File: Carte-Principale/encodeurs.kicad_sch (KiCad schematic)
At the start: 9 parts, among them J8 Encodeur_G, J9 Encodeur_D, U2 AM26LV32xD

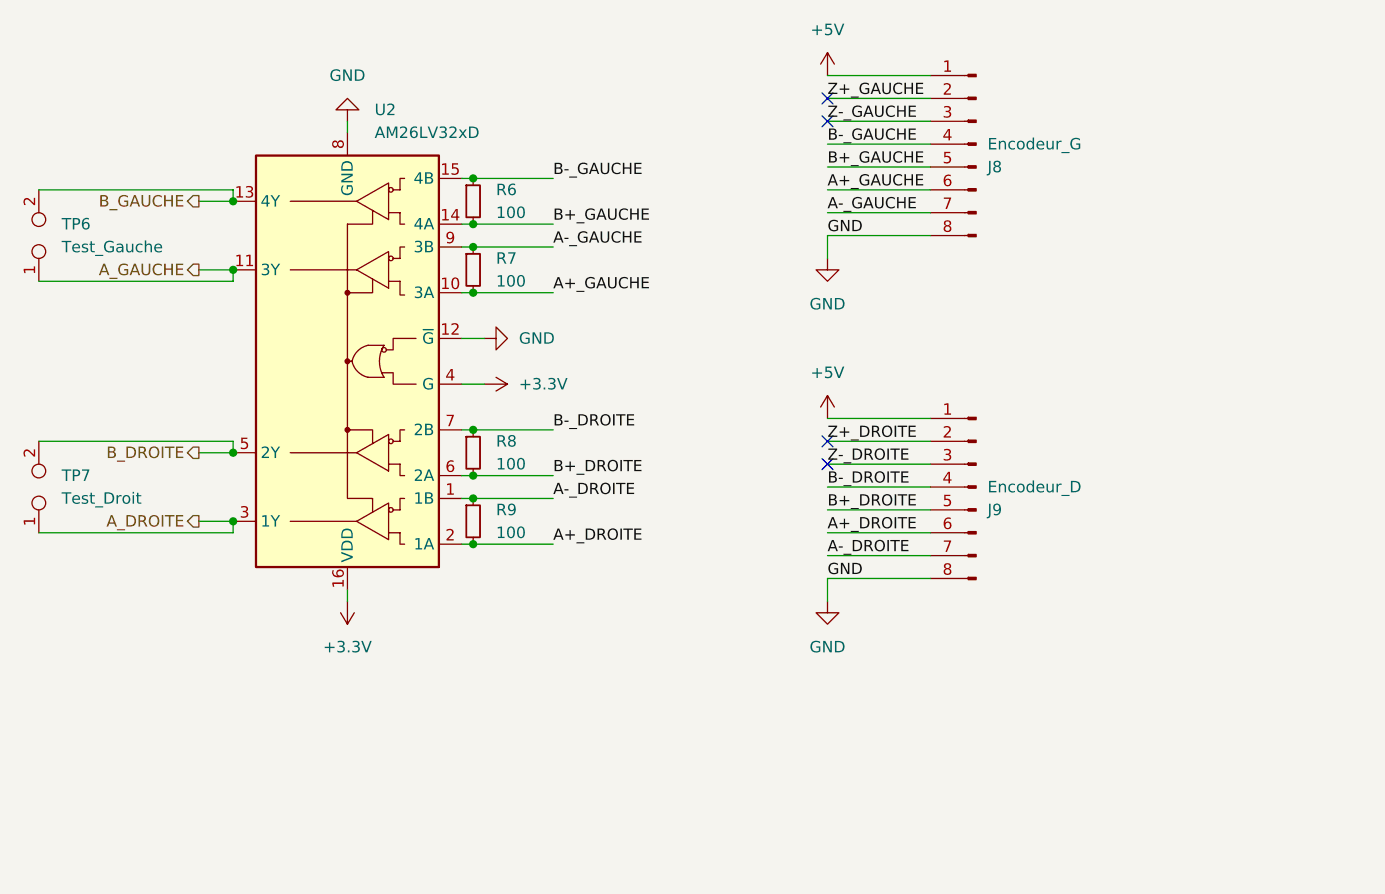
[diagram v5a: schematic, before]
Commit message: avancée
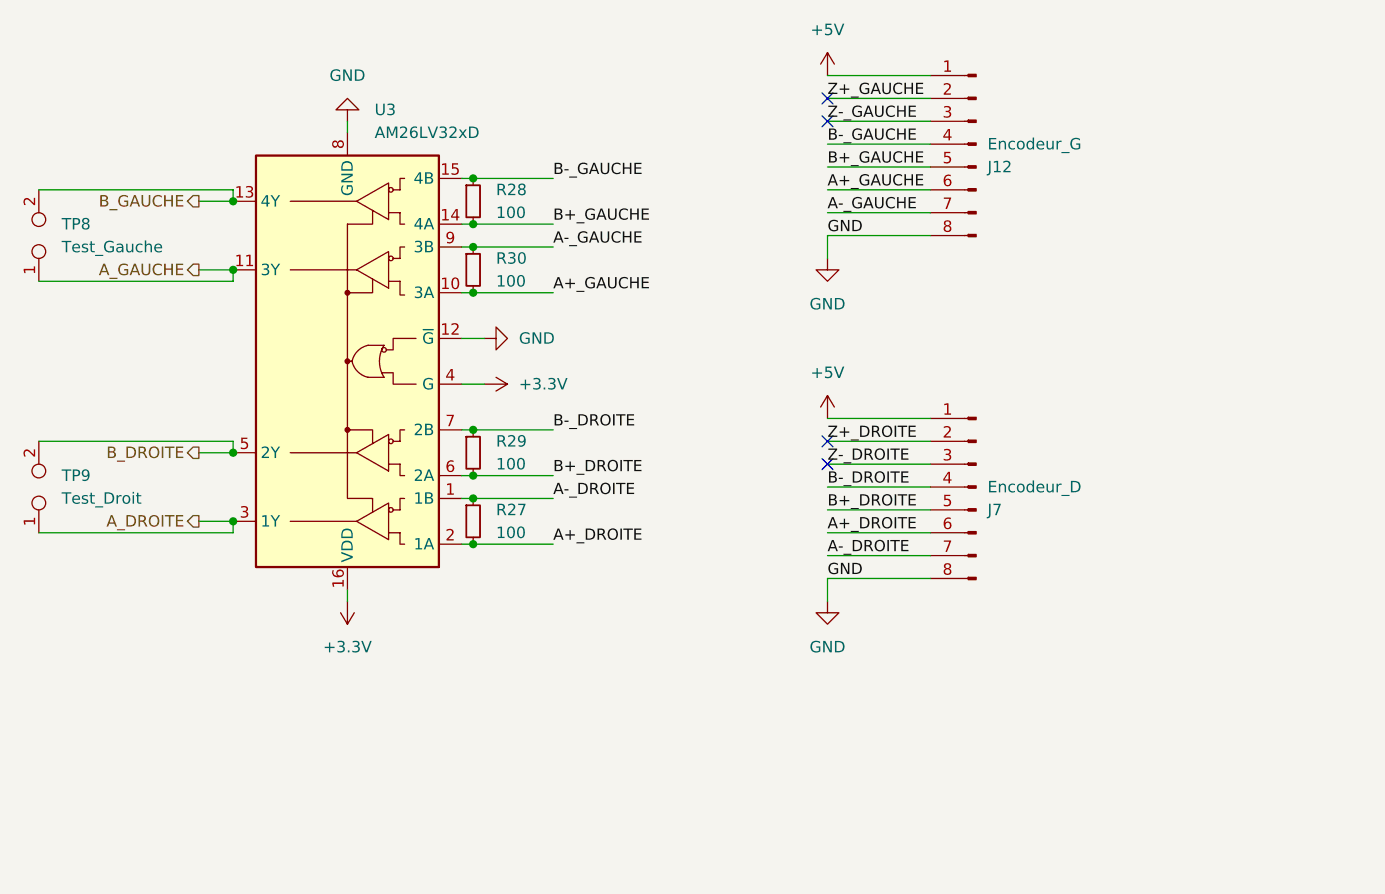
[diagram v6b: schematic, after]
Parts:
- renumbered J8 to J12, J9 to J7, R9 to R27, R6 to R28, R8 to R29, R7 to R30, TP6 to TP8, TP7 to TP9, U2 to U3
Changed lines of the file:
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@@
 		(dnp no)
 		(fields_autoplaced yes)
-		(property "Reference" "TP7"
+		(property "Reference" "TP9"
 			(at 40.64 77.4699 90)
 			(effects
@@
 			(project "Carte-Principale"
 				(path "/88b0dd29-ac24-4c5d-804c-fc642ecf6263/a2923913-7939-4f75-8694-93f1ab74a018"
-					(reference "TP7")
+					(reference "TP9")
 					(unit 1)
 				)
@@
 		(dnp no)
 		(fields_autoplaced yes)
-		(property "Reference" "J9"
+		(property "Reference" "J7"
 			(at 143.51 81.2801 0)
 			(effects
@@
 			(project "Carte-Principale"
 				(path "/88b0dd29-ac24-4c5d-804c-fc642ecf6263/a2923913-7939-4f75-8694-93f1ab74a018"
-					(reference "J9")
+					(reference "J7")
 					(unit 1)
 				)
@@
 		(dnp no)
 		(fields_autoplaced yes)
-		(property "Reference" "TP6"
+		(property "Reference" "TP8"
 			(at 40.64 49.5299 90)
 			(effects
@@
 			(project "Carte-Principale"
 				(path "/88b0dd29-ac24-4c5d-804c-fc642ecf6263/a2923913-7939-4f75-8694-93f1ab74a018"
-					(reference "TP6")
+					(reference "TP8")
 					(unit 1)
 				)
@@
 		(dnp no)
 		(fields_autoplaced yes)
-		(property "Reference" "R8"
+		(property "Reference" "R29"
 			(at 88.9 73.6599 0)
 			(effects
@@
 			(project "Carte-Principale"
 				(path "/88b0dd29-ac24-4c5d-804c-fc642ecf6263/a2923913-7939-4f75-8694-93f1ab74a018"
-					(reference "R8")
+					(reference "R29")
 					(unit 1)
 				)
@@
 		(dnp no)
 		(fields_autoplaced yes)
-		(property "Reference" "R7"
+		(property "Reference" "R30"
 			(at 88.9 53.3399 0)
 			(effects
@@
 			(project "Carte-Principale"
 				(path "/88b0dd29-ac24-4c5d-804c-fc642ecf6263/a2923913-7939-4f75-8694-93f1ab74a018"
-					(reference "R7")
+					(reference "R30")
 					(unit 1)
 				)
@@
 		(dnp no)
 		(fields_autoplaced yes)
-		(property "Reference" "J8"
+		(property "Reference" "J12"
 			(at 143.51 43.1801 0)
 			(effects
@@
 			(project "Carte-Principale"
 				(path "/88b0dd29-ac24-4c5d-804c-fc642ecf6263/a2923913-7939-4f75-8694-93f1ab74a018"
-					(reference "J8")
+					(reference "J12")
 					(unit 1)
 				)
@@
 		(dnp no)
 		(fields_autoplaced yes)
-		(property "Reference" "R6"
+		(property "Reference" "R28"
 			(at 88.9 45.7199 0)
 			(effects
@@
 			(project "Carte-Principale"
 				(path "/88b0dd29-ac24-4c5d-804c-fc642ecf6263/a2923913-7939-4f75-8694-93f1ab74a018"
-					(reference "R6")
+					(reference "R28")
 					(unit 1)
 				)
@@
 		(dnp no)
 		(fields_autoplaced yes)
-		(property "Reference" "R9"
+		(property "Reference" "R27"
 			(at 88.9 81.2799 0)
 			(effects
@@
 			(project "Carte-Principale"
 				(path "/88b0dd29-ac24-4c5d-804c-fc642ecf6263/a2923913-7939-4f75-8694-93f1ab74a018"
-					(reference "R9")
+					(reference "R27")
 					(unit 1)
 				)
@@
 		(dnp no)
 		(fields_autoplaced yes)
-		(property "Reference" "U2"
+		(property "Reference" "U3"
 			(at 75.4065 36.83 0)
 			(effects
@@
 			(project "Carte-Principale"
 				(path "/88b0dd29-ac24-4c5d-804c-fc642ecf6263/a2923913-7939-4f75-8694-93f1ab74a018"
-					(reference "U2")
-					(unit 1)
-				)
+					(reference "U3")
+					(unit 1)
+				)

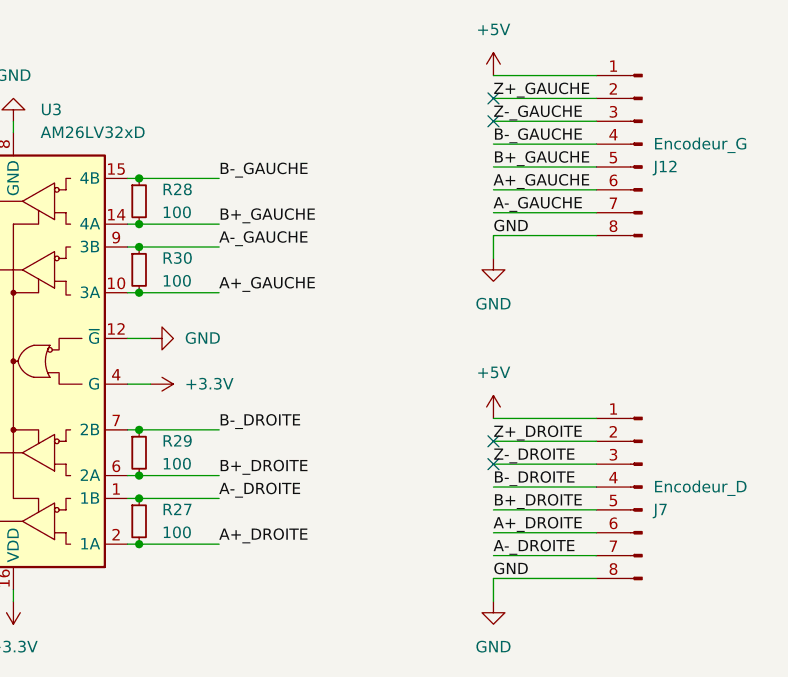
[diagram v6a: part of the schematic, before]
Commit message: Final pcb modification
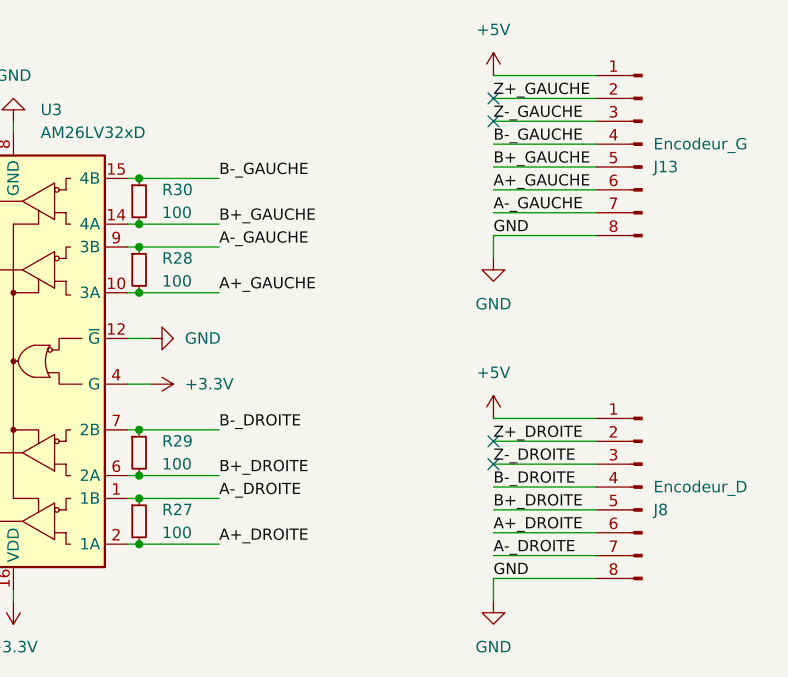
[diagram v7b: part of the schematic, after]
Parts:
- renumbered J12 to J13, J7 to J8, R30 to R28, R28 to R30
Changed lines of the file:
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@@
 		(dnp no)
 		(fields_autoplaced yes)
-		(property "Reference" "J7"
+		(property "Reference" "J8"
 			(at 143.51 81.2801 0)
 			(effects
@@
 			(project "Carte-Principale"
 				(path "/88b0dd29-ac24-4c5d-804c-fc642ecf6263/a2923913-7939-4f75-8694-93f1ab74a018"
-					(reference "J7")
+					(reference "J8")
 					(unit 1)
 				)
@@
 		(dnp no)
 		(fields_autoplaced yes)
-		(property "Reference" "R30"
+		(property "Reference" "R28"
 			(at 88.9 53.3399 0)
 			(effects
@@
 			(project "Carte-Principale"
 				(path "/88b0dd29-ac24-4c5d-804c-fc642ecf6263/a2923913-7939-4f75-8694-93f1ab74a018"
-					(reference "R30")
+					(reference "R28")
 					(unit 1)
 				)
@@
 		(dnp no)
 		(fields_autoplaced yes)
-		(property "Reference" "J12"
+		(property "Reference" "J13"
 			(at 143.51 43.1801 0)
 			(effects
@@
 			(project "Carte-Principale"
 				(path "/88b0dd29-ac24-4c5d-804c-fc642ecf6263/a2923913-7939-4f75-8694-93f1ab74a018"
-					(reference "J12")
+					(reference "J13")
 					(unit 1)
 				)
@@
 		(dnp no)
 		(fields_autoplaced yes)
-		(property "Reference" "R28"
+		(property "Reference" "R30"
 			(at 88.9 45.7199 0)
 			(effects
@@
 			(project "Carte-Principale"
 				(path "/88b0dd29-ac24-4c5d-804c-fc642ecf6263/a2923913-7939-4f75-8694-93f1ab74a018"
-					(reference "R28")
-					(unit 1)
-				)
+					(reference "R30")
+					(unit 1)
+				)

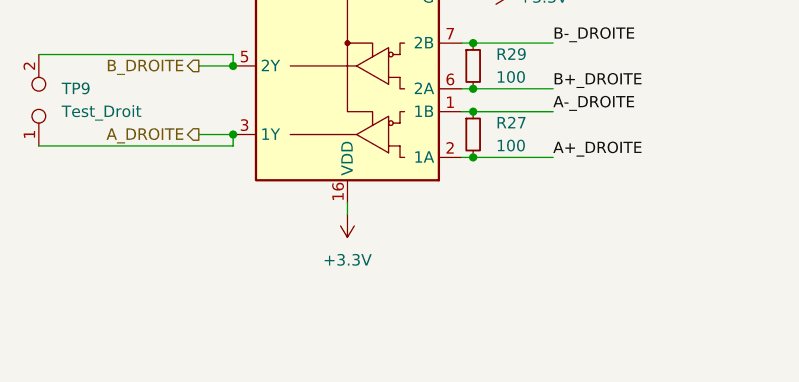
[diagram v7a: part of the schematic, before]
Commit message: Cartes élec à refaire et TODO
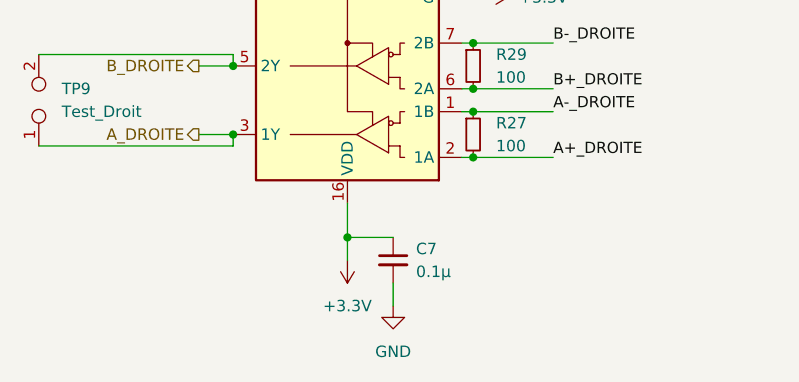
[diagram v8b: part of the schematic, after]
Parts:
- added C7: 0.1µ, Capacitor_SMD:C_1210_3225Metric_Pad1.33x2.70mm_HandSolder, symbol Device:C_Small
- J13, J8: footprint Connector_Molex:Molex_KK-254_AE-6410-08A_1x08_P2.54mm_Vertical -> Connector_JST:JST_XH_B8B-XH-A_1x08_P2.50mm_Vertical
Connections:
- net +3.3V: now also C7.1
- net GND: now also C7.2
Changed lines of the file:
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@@
+		(color 0 0 0 0)
+	)
+	(junction
+		(at 72.39 93.98)
+		(diameter 0)
 		(color 0 0 0 0)
 	)
@@
 	(wire
 		(pts
+			(xy 77.47 99.06) (xy 77.47 101.6)
+		)
+		(stroke
+			(width 0)
+			(type default)
+		)
+	)
+	(wire
+		(pts
 			(xy 87.63 62.23) (xy 85.09 62.23)
 		)
@@
 	(wire
 		(pts
+			(xy 72.39 93.98) (xy 72.39 90.17)
+		)
+		(stroke
+			(width 0)
+			(type default)
+		)
+	)
+	(wire
+		(pts
 			(xy 137.16 33.02) (xy 125.73 33.02)
 		)
@@
 	(wire
 		(pts
-			(xy 72.39 91.44) (xy 72.39 90.17)
+			(xy 72.39 96.52) (xy 72.39 93.98)
 		)
 		(stroke
@@
 		(pts
 			(xy 95.25 85.09) (xy 86.36 85.09)
+		)
+		(stroke
+			(width 0)
+			(type default)
+		)
+	)
+	(wire
+		(pts
+			(xy 72.39 93.98) (xy 77.47 93.98)
 		)
 		(stroke
@@
 			)
 		)
-		(property "Footprint" "Connector_Molex:Molex_KK-254_AE-6410-08A_1x08_P2.54mm_Vertical"
+		(property "Footprint" "Connector_JST:JST_XH_B8B-XH-A_1x08_P2.50mm_Vertical"
 			(at 142.24 78.74 0)
 			(effects
@@
 				(path "/88b0dd29-ac24-4c5d-804c-fc642ecf6263/a2923913-7939-4f75-8694-93f1ab74a018"
 					(reference "TP8")
+					(unit 1)
+				)
+			)
+		)
+	)
+	(symbol
+		(lib_id "power:GND")
+		(at 77.47 101.6 0)
+		(unit 1)
+		(exclude_from_sim no)
+		(in_bom yes)
+		(on_board yes)
+		(dnp no)
+		(fields_autoplaced yes)
+		(property "Reference" "#PWR011"
+			(at 77.47 107.95 0)
+			(effects
+				(font
+					(size 1.27 1.27)
+				)
+				(hide yes)
+			)
+		)
+		(property "Value" "GND"
+			(at 77.47 106.68 0)
+			(effects
+				(font
+					(size 1.27 1.27)
+				)
+			)
+		)
+		(property "Footprint" ""
+			(at 77.47 101.6 0)
+			(effects
+				(font
+					(size 1.27 1.27)
+				)
+				(hide yes)
+			)
+		)
+		(property "Datasheet" ""
+			(at 77.47 101.6 0)
+			(effects
+				(font
+					(size 1.27 1.27)
+				)
+				(hide yes)
+			)
+		)
+		(property "Description" "Power symbol creates a global label with name \"GND\" , ground"
+			(at 77.47 101.6 0)
+			(effects
+				(font
+					(size 1.27 1.27)
+				)
+				(hide yes)
+			)
+		)
+		(pin "1"
+		)
+		(instances
+			(project "Carte-Principale"
+				(path "/88b0dd29-ac24-4c5d-804c-fc642ecf6263/a2923913-7939-4f75-8694-93f1ab74a018"
+					(reference "#PWR011")
 					(unit 1)
 				)
@@
 			)
 		)
-		(property "Footprint" "Connector_Molex:Molex_KK-254_AE-6410-08A_1x08_P2.54mm_Vertical"
+		(property "Footprint" "Connector_JST:JST_XH_B8B-XH-A_1x08_P2.50mm_Vertical"
 			(at 142.24 40.64 0)
 			(effects
@@
 	(symbol
 		(lib_id "power:+3.3V")
-		(at 72.39 91.44 180)
+		(at 72.39 96.52 180)
 		(unit 1)
 		(exclude_from_sim no)
@@
 		(fields_autoplaced yes)
 		(property "Reference" "#PWR033"
-			(at 72.39 87.63 0)
+			(at 72.39 92.71 0)
 			(effects
 				(font
@@
 		)
 		(property "Value" "+3.3V"
+			(at 72.39 101.6 0)
+			(effects
+				(font
+					(size 1.27 1.27)
+				)
+			)
+		)
+		(property "Footprint" ""
 			(at 72.39 96.52 0)
 			(effects
@@
 					(size 1.27 1.27)
 				)
-			)
-		)
-		(property "Footprint" ""
-			(at 72.39 91.44 0)
-			(effects
-				(font
-					(size 1.27 1.27)
-				)
 				(hide yes)
 			)
 		)
 		(property "Datasheet" ""
-			(at 72.39 91.44 0)
+			(at 72.39 96.52 0)
 			(effects
 				(font
@@
 		)
 		(property "Description" "Power symbol creates a global label with name \"+3.3V\""
-			(at 72.39 91.44 0)
+			(at 72.39 96.52 0)
 			(effects
 				(font
@@
 					(unit 1)
 				)
+			)
+		)
+	)
+	(symbol
+		(lib_id "Device:C_Small")
+		(at 77.47 96.52 0)
+		(unit 1)
+		(exclude_from_sim no)
+		(in_bom yes)
+		(on_board yes)
+		(dnp no)
+		(fields_autoplaced yes)
+		(property "Reference" "C7"
+			(at 80.01 95.2562 0)
+			(effects
+				(font
+					(size 1.27 1.27)
+				)
+				(justify left)
+			)
+		)
+		(property "Value" "0.1µ"
+			(at 80.01 97.7962 0)
+			(effects
+				(font
+					(size 1.27 1.27)
+				)
+				(justify left)
+			)
+		)
+		(property "Footprint" "Capacitor_SMD:C_1210_3225Metric_Pad1.33x2.70mm_HandSolder"
+			(at 77.47 96.52 0)
+			(effects
+				(font
+					(size 1.27 1.27)
+				)
+				(hide yes)
+			)
+		)
+		(property "Datasheet" "~"
+			(at 77.47 96.52 0)
+			(effects
+				(font
+					(size 1.27 1.27)
+				)
+				(hide yes)
+			)
+		)
+		(property "Description" "Unpolarized capacitor, small symbol"
+			(at 77.47 96.52 0)
+			(effects
+				(font
+					(size 1.27 1.27)
+				)
+				(hide yes)
+			)
+		)
+		(pin "2"
+		)
+		(pin "1"
+		)
+		(instances
+			(project "Carte-Principale"
+				(path "/88b0dd29-ac24-4c5d-804c-fc642ecf6263/a2923913-7939-4f75-8694-93f1ab74a018"
+					(reference "C7")
+					(unit 1)
+				)
